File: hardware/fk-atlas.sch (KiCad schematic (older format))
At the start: 68 parts, among them J1 CONN_02x05_SWD, J10 CONN_01x04, J2 MICRO-USB-VERT-TOP, J3 CONN_01x02, J4 CONN_01x03_SERIAL, J5 CONN_01x05, J6 CONN_01x04, J7 CONN_01x05, J8 CONN_01x02, J9 MICRO-USB-HORIZ-BOTTOM, M1 MOUNT_HOLE, M2 MOUNT_HOLE, M3 MOUNT_HOLE, M4 MOUNT_HOLE, M5 FIDUCIAL, M6 FIDUCIAL, M7 FIDUCIAL, Q4 2N7002LT1G, SW1 SPNO, U1 S25FL116K0XMFI041, U2 ATSAMD21G18A-AU, U3 MCP1700T-3302E/MB, U4 TPS2052B, U5 SK6812, Y1 FC-135

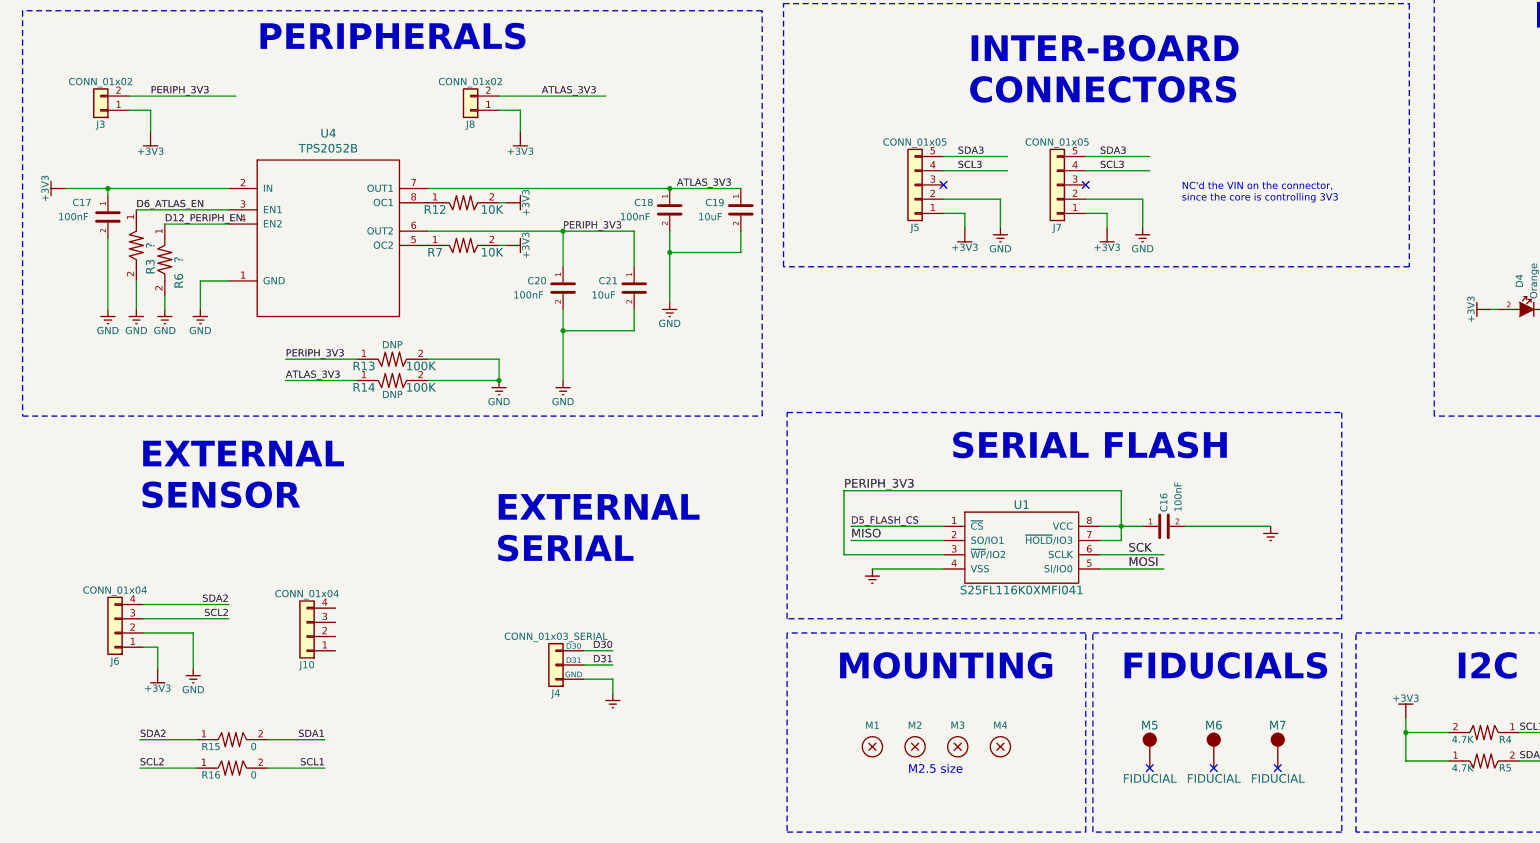
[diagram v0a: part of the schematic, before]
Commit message: Finished DRC check, no errors
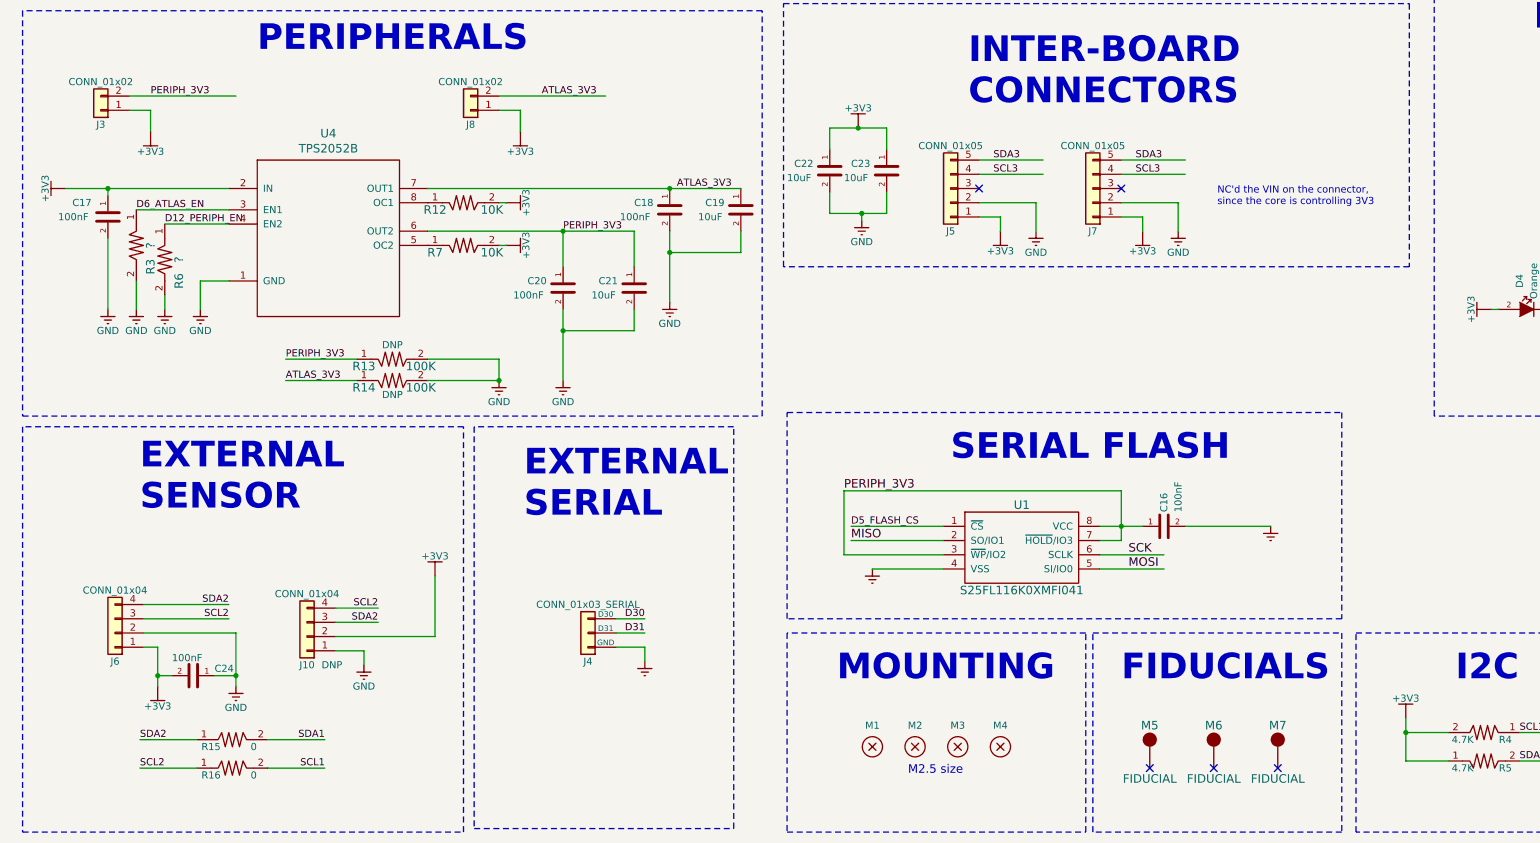
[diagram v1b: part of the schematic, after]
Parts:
- added C22, C23: 10uF, conservify:CAP-0603, symbol fk-atlas-rescue:CAPACITOR_CERAMIC-conservify
- added C24: 100nF, conservify:CAP-0603, symbol fk-atlas-rescue:CAPACITOR_CERAMIC-conservify
- J10: footprint conservify:Molex_CLIK-Mate_502382-0470_1x04_P1.25mm_Vertical -> conservify:BM04B-SRSS-TB; Population (none) -> DNP
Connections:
- wire segments 303 -> 322
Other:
- moved on the sheet: J4, J5, J7
